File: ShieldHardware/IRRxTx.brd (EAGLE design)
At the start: 48.6 x 49.3 mm, 23 parts, among them IC1 ATMEGA8, J2 Analogs, J4 D8_D13, J5 D0..D7, Q1 16Mhz

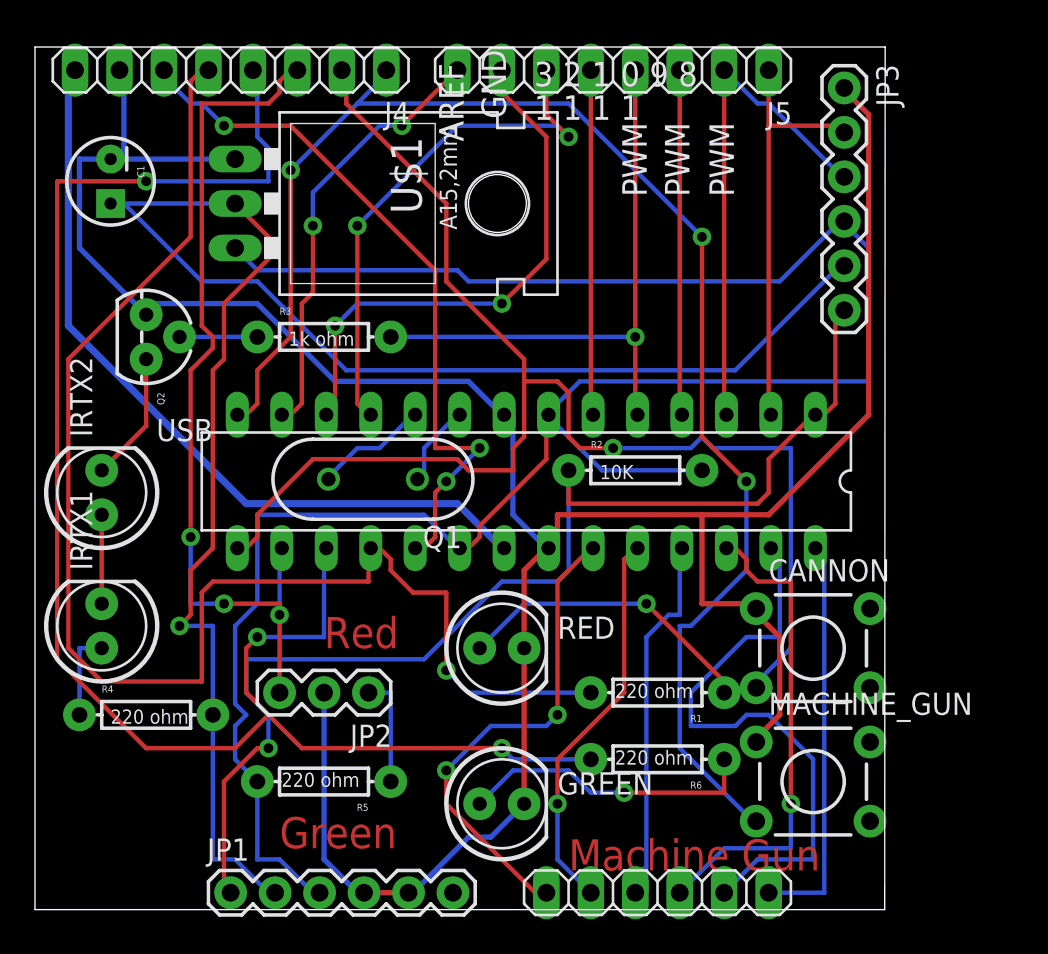
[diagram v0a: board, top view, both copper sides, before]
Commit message: v.0.07
Added Grenade
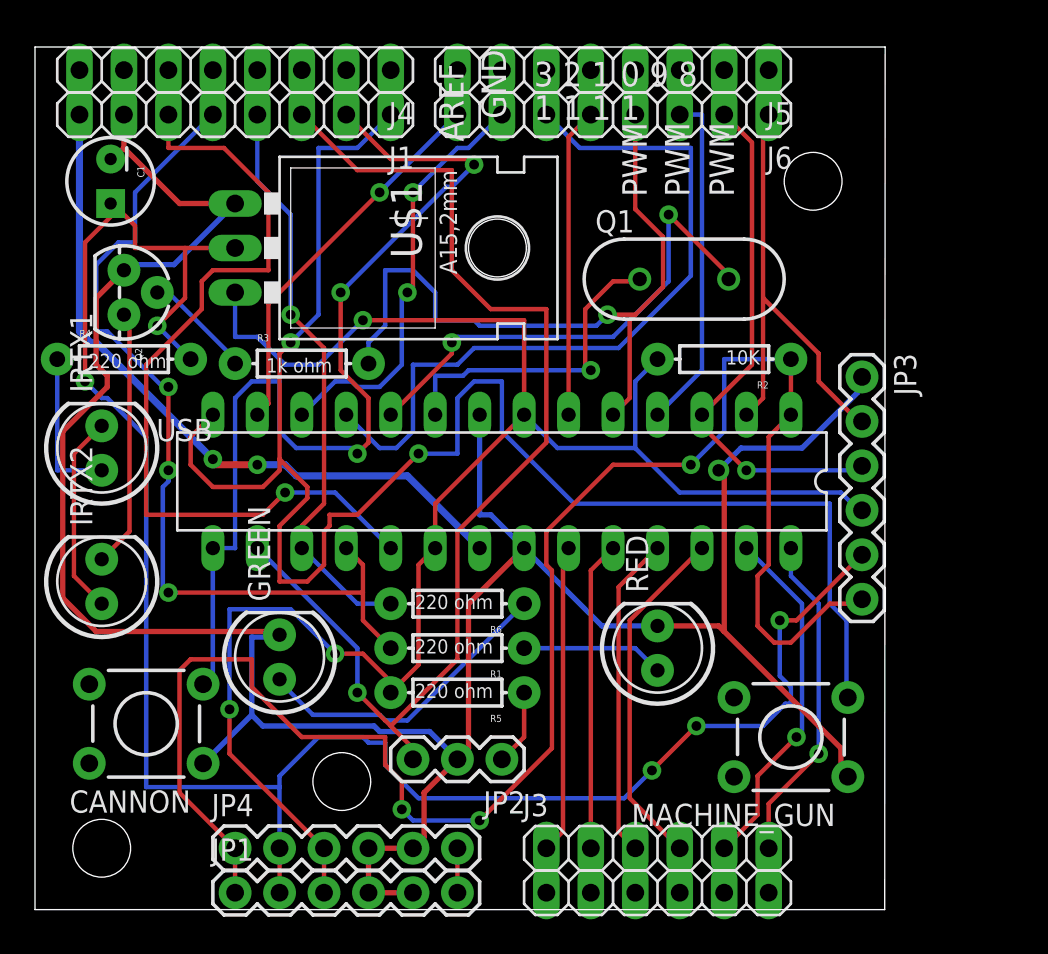
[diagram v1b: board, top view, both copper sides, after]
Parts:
- added J1: D8_D13, pinhead:1X08
- added J3: Analogs, pinhead:1X06
- added J6: D0..D7, pinhead:1X08
- added JP4: Power_Gnd, SparkFun:1X06
- added U$2, U$3, U$4: (no value), SparkFun:STAND-OFF
- moved CANNON 38.3 mm to (6.35, 10.9), turned to 180 degrees
- moved Q1 21.1 mm to (37.1, 36.3), turned to 0 degrees
- moved R4 20.4 mm to (5.08, 31.8)
- moved JP3 16.5 mm to (47.2, 30.7)
- moved GREEN 15.2 mm to (14.0, 14.7), turned to 90 degrees
- moved R6 14.5 mm to (24.1, 17.8)
- moved R1 11.7 mm to (24.1, 15.2)
- moved IRTX1 10.2 mm to (3.81, 26.7)
- moved R5 9.16 mm to (24.1, 12.7)
- moved RED 8.89 mm to (35.6, 15.2), turned to 90 degrees
- moved JP2 8.52 mm to (26.7, 8.89)
- moved R2 8.13 mm to (39.4, 31.8), turned to 180 degrees
- moved IRTX2 5.08 mm to (3.81, 19.1)
- moved MACHINE_GUN 2.84 mm to (43.2, 10.2), turned to 180 degrees
- moved Q2 2.84 mm to (5.08, 35.6)
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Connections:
- new net N$10: JP1.6, JP4.6
- net 3.3V: now also JP4.2
- net AREF: now also J1.8
- net D0: now also J6.1
- net D1: now also J6.2
- net D10: now also J1.3
- net D11: now also J1.4
- net D12: now also J1.5
- net D13: now also J1.6
- net D18: now also J3.5
- net D2: now also J6.3
- net D3: now also J6.4
- net D4: now also J6.5
- net D5: now also J6.6
- net D6: now also J6.7
- net D7: now also J6.8
- net D8: now also J1.1
- net D9: now also J1.2
- net GND: now also J1.7, JP4.4, JP4.5
- net N$16: now also J3.1
- net N$17: now also J3.2
- net N$18: now also J3.3
- net N$19: now also J3.4
- net N$21: now also J3.6
- net RST: now also JP4.1
- net VCC: now also JP4.3
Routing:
- net D11: track 94.9 -> 35.8 mm, vias 3 -> 1
- net RST: track 68.2 -> 100.3 mm, vias 1 -> 3
- net D12: track 80.8 -> 53.8 mm, vias 1 -> 3
- net VCC: track 124.2 -> 102.1 mm, vias 0 -> 3
- net N$1: track 6.52 -> 28.3 mm, vias 0 -> 2
- net D9: track 79.8 -> 60.8 mm, vias 1 -> 3
- net D10: track 50.1 -> 67.7 mm, vias 3 -> 1
- net D5: track 30.2 -> 45.7 mm, vias 2 -> 0
- net D8: track 85.0 -> 100.0 mm, vias 3 -> 2
- net N$2: track 4.73 -> 18.7 mm, vias 0 -> 1
- net 3.3V: track 101.2 -> 112.8 mm, vias 1 -> 5
- net D18: track 33.8 -> 23.0 mm, vias 0 -> 1
- net D3: track 33.8 -> 44.1 mm
- net N$3: track 17.5 -> 8.15 mm, vias 1 -> 0
- net D13: track 41.2 -> 50.2 mm, vias 3 -> 1
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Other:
- board text removed: "Green"
- board text removed: "Machine Gun"
- board text removed: "Red"
